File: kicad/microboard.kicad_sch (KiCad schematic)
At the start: 10 parts, among them J2 to microboard, J3 to baseboard, Q1 AH3712-P-B, U5 LM35-LP

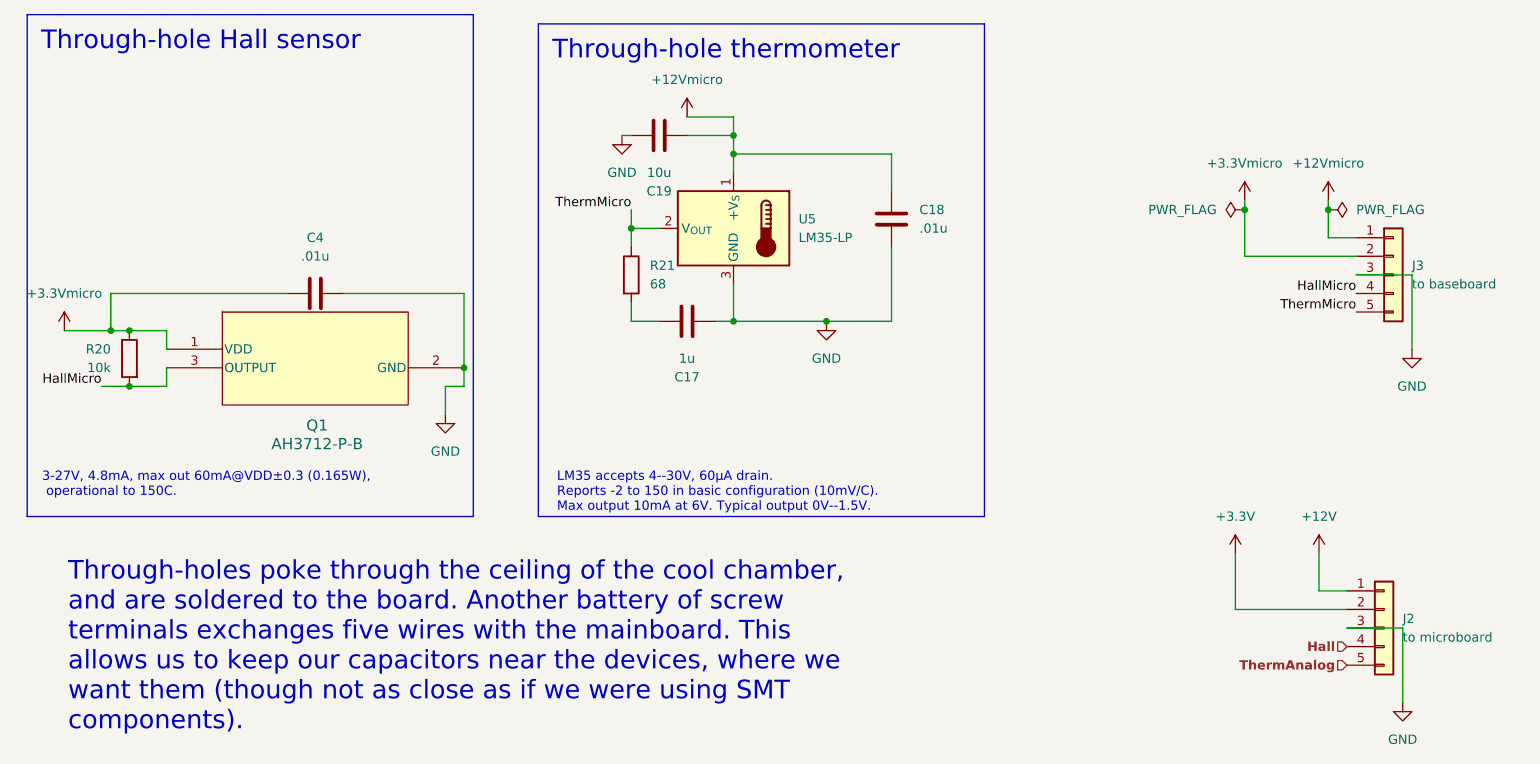
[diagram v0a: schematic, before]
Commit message: [schematics] sync to grid
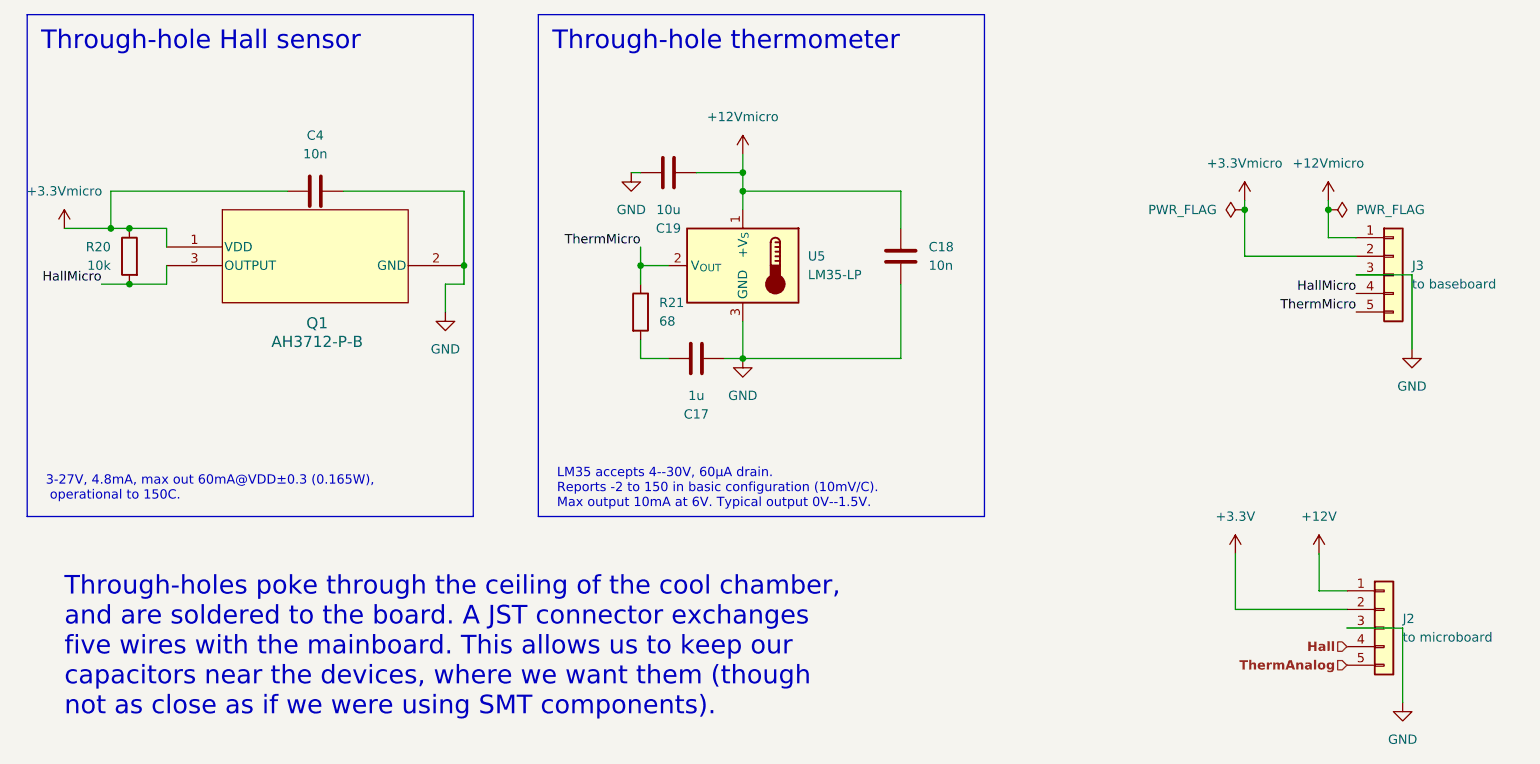
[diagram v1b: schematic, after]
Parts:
- C18, C4: value .01u -> 10n
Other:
- note added: "Through-holes poke through the ceiling of the cool chamber, and are soldered to the board. A JST connector exchanges five wires with the mainboard. This allows us to keep our capacitors near the devices, where we want them (though not as close as if we were using SMT components)."
- note removed: "Through-holes poke through the ceiling of the cool chamber, and are soldered to the board. Another battery of screw terminals exchanges five wires with the mainboard. This allows us to keep our capacitors near the devices, where we want them (though not as close as if we were using SMT components)."
- moved on the sheet: C17, C18, C19, C4, Q1, R20, R21, U5

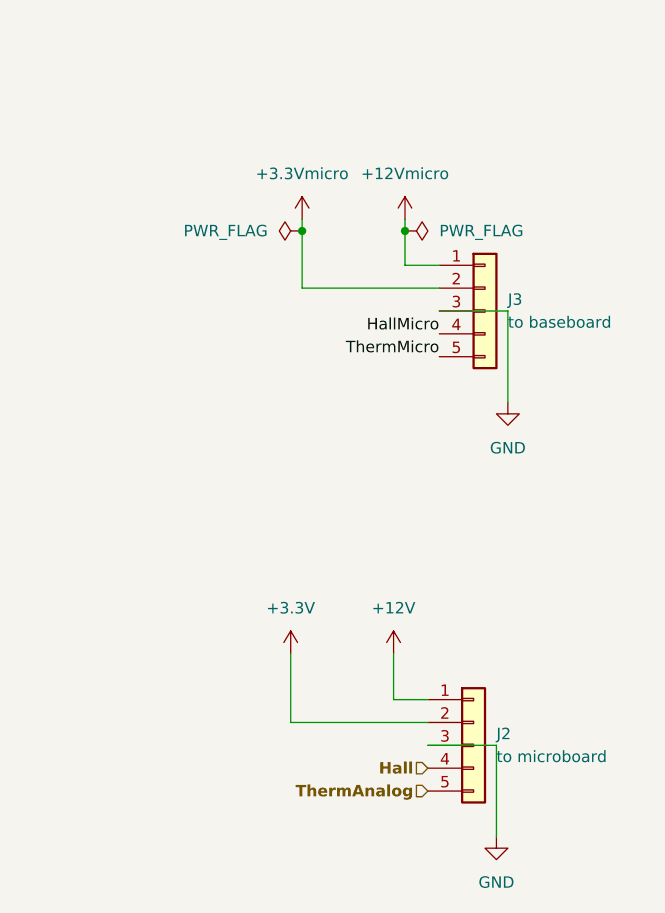
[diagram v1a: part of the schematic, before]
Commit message: [kicad] tighten things up
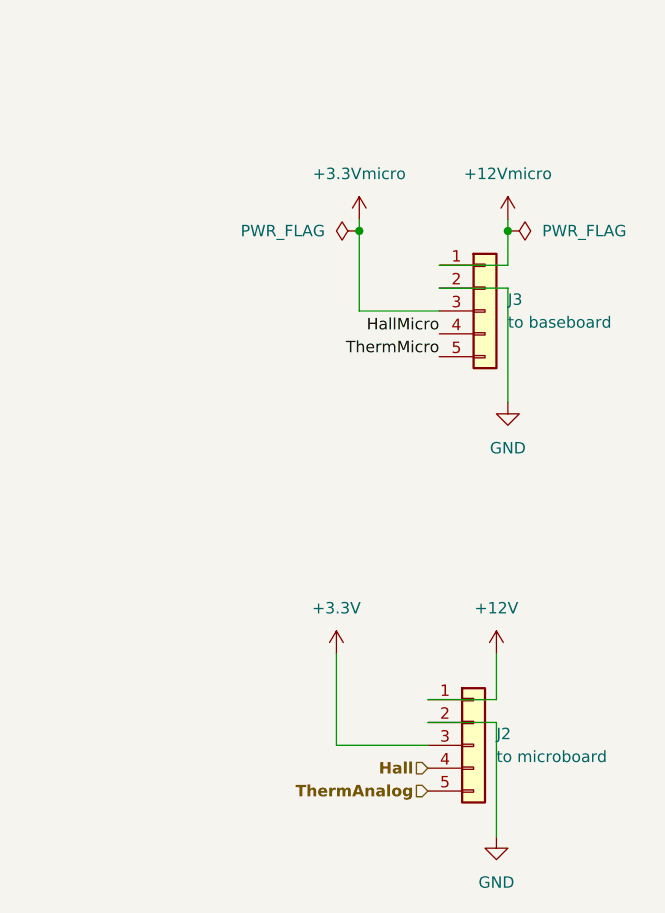
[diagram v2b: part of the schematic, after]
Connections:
- net +3.3V: now also J2.3 (Pin_3); no longer J2.2 (Pin_2)
- net +3.3Vmicro: now also J3.3 (Pin_3); no longer J3.2 (Pin_2)
- net GND: now also J2.2 (Pin_2), J3.2 (Pin_2); no longer J2.3 (Pin_3), J3.3 (Pin_3)
